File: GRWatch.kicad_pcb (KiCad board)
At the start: 2 copper layers, 35 x 35 mm, 20 parts, among them J1 JST_SH_06, U1 R5F100LJAFB, U2 MULTI_SW, U3 SSD1306, U5 BUZZER, Y1 32.768k

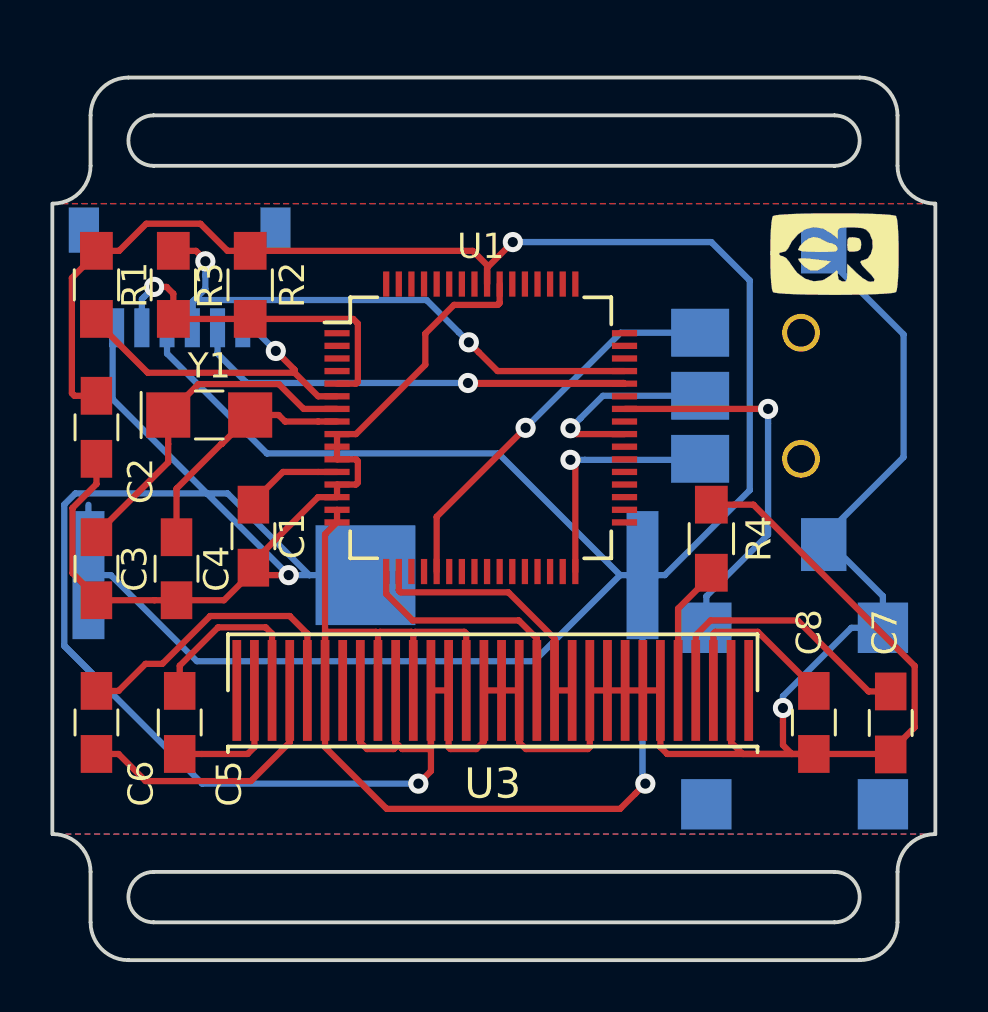
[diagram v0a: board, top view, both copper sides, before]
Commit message: add tiny version
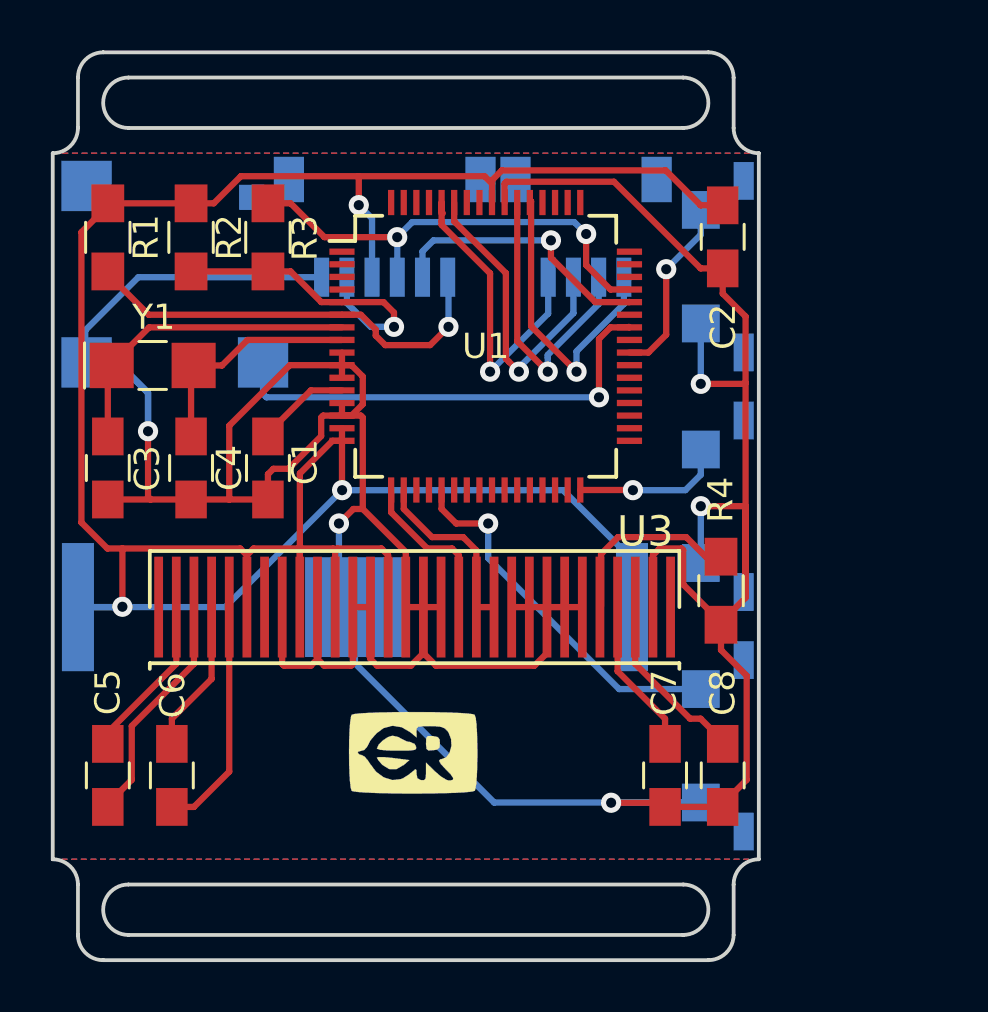
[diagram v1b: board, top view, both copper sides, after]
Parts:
- removed U5: BUZZER, misc:BZ7025
- added J2: JST_SH_04, JST-SH:JST-SM-04B-SRSS-TB, B.Cu at (116.4, 91.7)
- added SW1: SW_Push, misc:THAM16, B.Cu at (122.2, 102.7)
- added SW2: SW_Push, misc:THAM16, B.Cu at (122.2, 93.2)
- added SW3: SW_Push, misc:THAM16, B.Cu at (122.2, 112.2)
- U2: value MULTI_SW -> BUZZER; footprint misc:TST-1005 -> misc:BZ7025_3pin
- moved C2 26.0 mm to (121.8, 92.0)
- moved G*** 25.9 mm to (109.5, 112.4)
- moved U2 25.3 mm to (100.1, 93.4), turned to 0 degrees
- moved C7 9.19 mm to (119.5, 113.3)
- moved J1 8.37 mm to (108.4, 91.7)
- moved U3 4.53 mm to (109.6, 106.7)
- moved R3 4.20 mm to (103.8, 92.0)
- moved C8 4.18 mm to (121.8, 113.3)
- moved C4 4.04 mm to (100.7, 101.1)
- moved C3 4.02 mm to (97.4, 101.1)
- moved C6 3.65 mm to (100.0, 113.3), turned to 270 degrees
- moved C5 3.54 mm to (97.4, 113.3), turned to 270 degrees
- moved U1 3.24 mm to (112.4, 96.3)
- moved R2 3.01 mm to (100.7, 92.0)
- moved Y1 2.98 mm to (99.2, 97.1)
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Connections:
- J1 pad M1: Net-(J1-PadM1) -> (no net)
- J1 pad M2: Net-(J1-PadM2) -> (no net)
- U1 pad 1: Net-(U1-Pad1) -> (no net)
- U1 pad 19: Net-(U1-Pad19) -> (no net)
- U1 pad 2: Net-(U1-Pad2) -> (no net)
- U1 pad 20: Net-(U1-Pad20) -> (no net)
- U1 pad 22: Net-(U1-Pad22) -> (no net)
- U1 pad 23: Net-(U1-Pad23) -> (no net)
- U1 pad 24: Net-(U1-Pad24) -> (no net)
- U1 pad 25: Net-(U1-Pad25) -> (no net)
- U1 pad 26: Net-(U1-Pad26) -> (no net)
- U1 pad 27: Net-(U1-Pad27) -> (no net)
- U1 pad 28: Net-(U1-Pad28) -> (no net)
- U1 pad 29: Net-(U1-Pad29) -> (no net)
- U1 pad 3: Net-(U1-Pad3) -> (no net)
- U1 pad 30: Net-(U1-Pad30) -> (no net)
- U1 pad 31: Net-(U1-Pad31) -> (no net)
- U1 pad 33: Net-(U1-Pad33) -> (no net)
- U1 pad 34: Net-(U1-Pad34) -> (no net)
- U1 pad 35: Net-(U1-Pad35) -> (no net)
- U1 pad 36: Net-(U1-Pad36) -> (no net)
- U1 pad 37: Net-(U1-Pad37) -> (no net)
- U1 pad 38: Net-(U1-Pad38) -> (no net)
- U1 pad 39: Net-(U1-Pad39) -> (no net)
- U1 pad 4: Net-(U1-Pad4) -> (no net)
- U1 pad 41: Net-(U1-Pad41) -> (no net)
- U1 pad 43: Net-(U1-Pad43) -> (no net)
- U1 pad 46: Net-(U1-Pad46) -> (no net)
- U1 pad 47: Net-(U1-Pad47) -> (no net)
- U1 pad 48: Net-(U1-Pad48) -> (no net)
- U1 pad 49: Net-(U1-Pad49) -> (no net)
- U1 pad 50: Net-(U1-Pad50) -> (no net)
- U1 pad 51: Net-(U1-Pad51) -> (no net)
- U1 pad 52: Net-(U1-Pad52) -> (no net)
- U1 pad 53: Net-(U1-Pad53) -> A1
- U1 pad 54: Net-(U1-Pad54) -> A0
- U1 pad 57: Net-(U1-Pad57) -> (no net)
- U1 pad 58: Net-(U1-Pad58) -> (no net)
- U1 pad 59: Net-(U1-Pad59) -> D8
- U1 pad 60: Net-(U1-Pad60) -> D7
- U1 pad 61: Net-(U1-Pad61) -> (no net)
- U1 pad 62: Net-(U1-Pad62) -> (no net)
- U1 pad 63: Net-(U1-Pad63) -> (no net)
- U1 pad 64: Net-(U1-Pad64) -> (no net)
- U2 pad 1: SW1 -> Net-(U1-Pad42)
- U2 pad 2: SW2 -> GND
- U2 pad 3: SW3 -> (no net)
- U2 pad 4: GND -> (no net)
- U3 pad 1: Net-(U3-Pad1) -> (no net)
- U3 pad 30: Net-(U3-Pad30) -> (no net)
- U3 pad 7: Net-(U3-Pad7) -> (no net)
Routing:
- net +3V3: track 148.1 -> 108.5 mm, vias 2 -> 3
- net RXD: track 23.9 -> 10.8 mm
- net A1: track 0.00 -> 12.7 mm, vias 0 -> 1
- net D7: track 0.00 -> 12.6 mm, vias 0 -> 1
- net A0: track 0.00 -> 12.4 mm, vias 0 -> 1
- net D8: track 0.00 -> 12.4 mm, vias 0 -> 1
- net GND: track 176.4 -> 170.1 mm, vias 3 -> 5
- net TXD: track 23.7 -> 18.6 mm
- net Net-(C7-Pad1): track 11.3 -> 6.20 mm
- net Net-(C6-Pad1): track 10.8 -> 6.08 mm
- net SW1: track 9.87 -> 6.04 mm
- net DTR: track 13.7 -> 17.2 mm
- net SCL: track 9.65 -> 6.33 mm
- net SDA: track 10.5 -> 7.26 mm
- net Net-(U1-Pad42): track 15.4 -> 18.4 mm
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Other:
- board size 35 x 35 mm -> 28 x 36 mm
